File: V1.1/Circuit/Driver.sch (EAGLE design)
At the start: 25 parts, among them IC1 DRV8300DIPWR

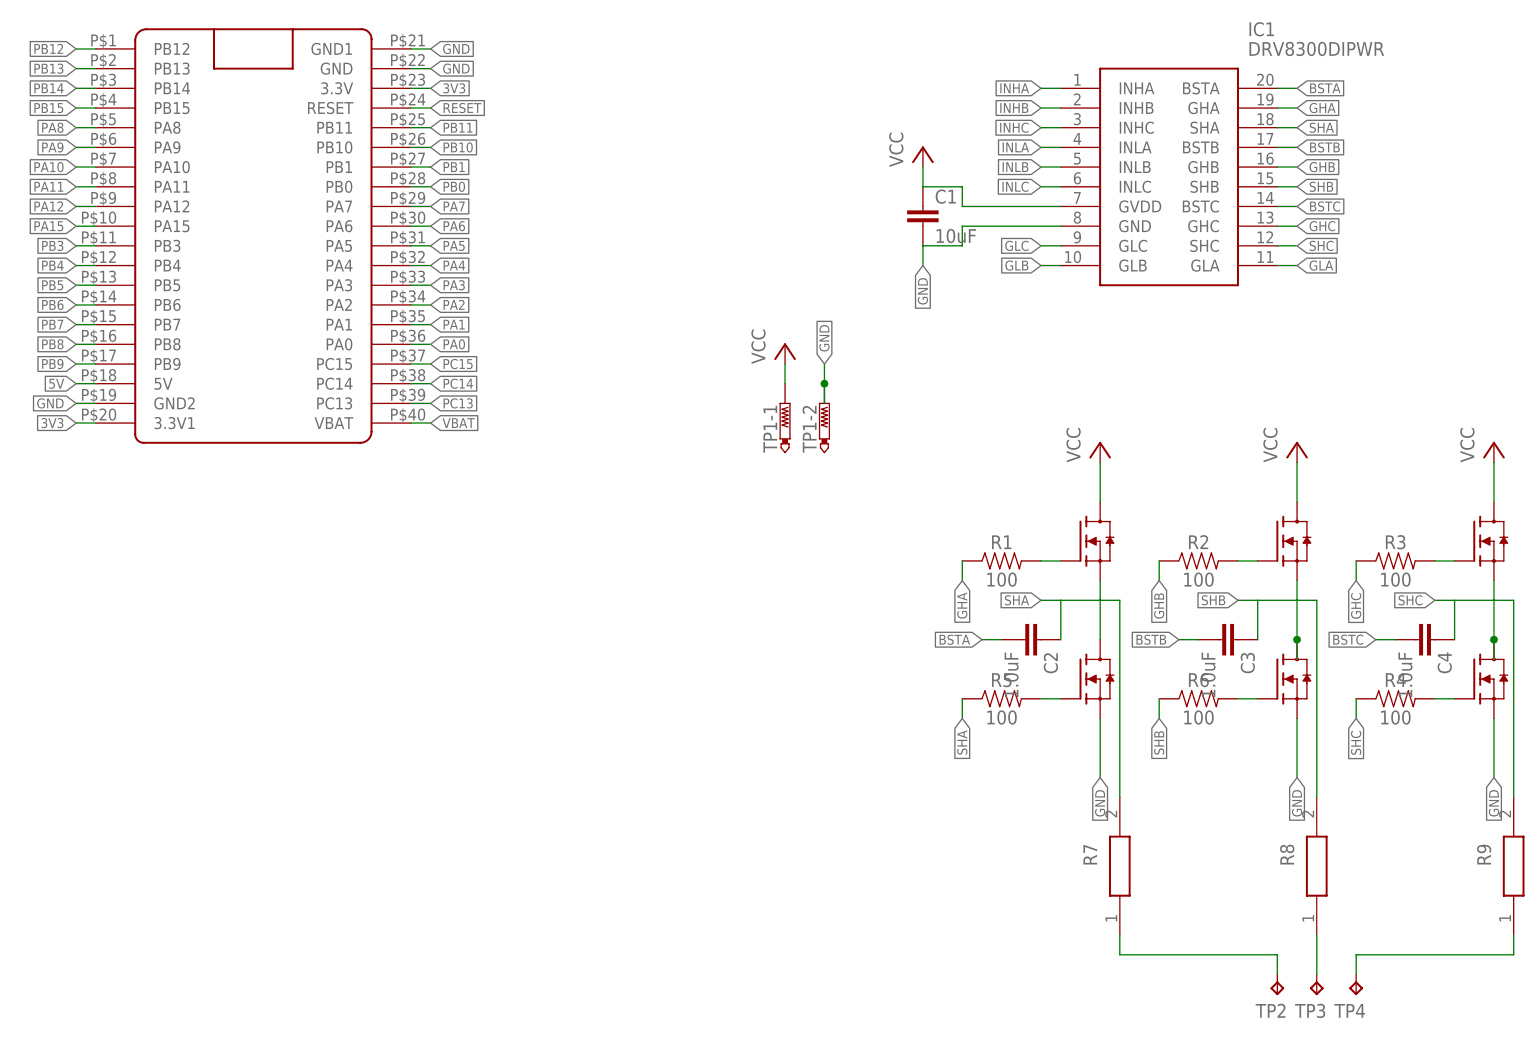
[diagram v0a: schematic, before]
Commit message: Added the FOC library
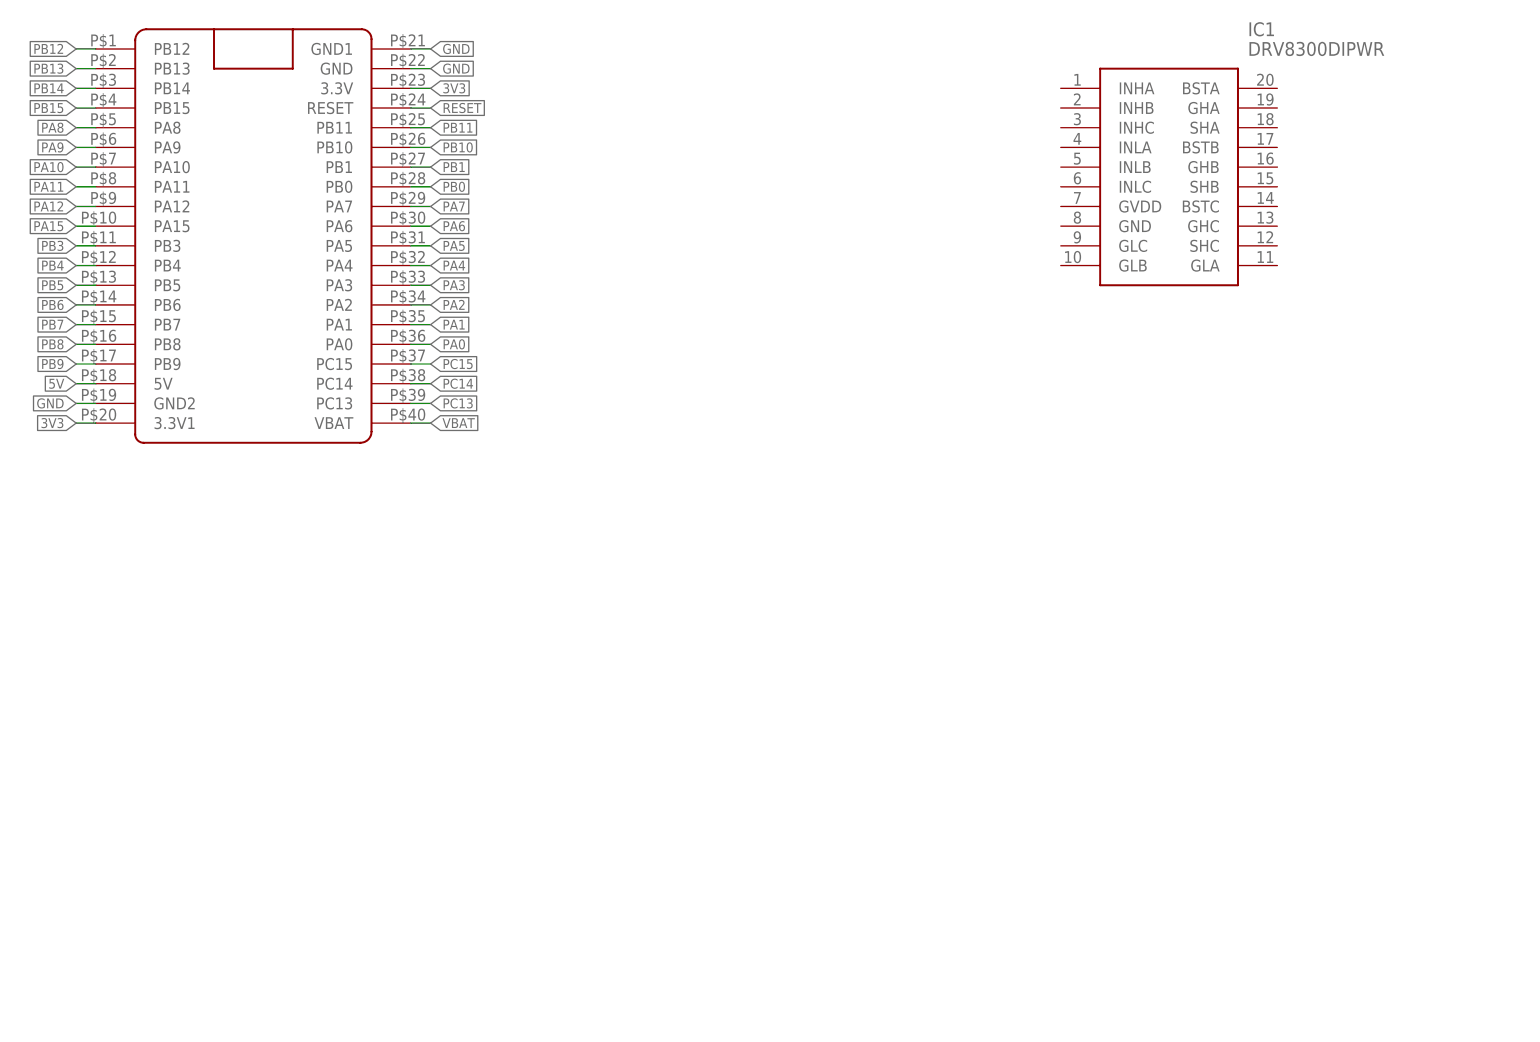
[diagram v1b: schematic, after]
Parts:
- removed C1: 10uF, SparkFun-Capacitors:10UF-0603-6.3V-20%
- removed C2, C3, C4: 1.0uF, SparkFun-Capacitors:1.0UF-0603-16V-10%
- removed R1, R2, R3, R4, R5, R6: 100, SparkFun-Resistors:100OHM-0603-1/10W-1%
- removed R7, R8, R9: CR2512-FX-51R1ELF, CR2512-FX-51R1ELF:CR2512-FX-51R1ELF
- removed TP1: PTR2, testpad:PTR2
- removed TP2, TP3, TP4: TPTP20SQ, testpad:TPTP20SQ
- removed U$2, U$3, U$4, U$5, U$6, U$7: IRLR7843, BLDC project:IRLR7843
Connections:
- removed net BSTA: C2.2, IC1.BSTA
- removed net BSTB: C3.2, IC1.BSTB
- removed net BSTC: C4.2, IC1.BSTC
- removed net GHA: IC1.GHA, R1.1
- removed net GHB: IC1.GHB, R2.1
- removed net GHC: IC1.GHC, R3.1
- removed net GLA: IC1.GLA
- removed net GLB: IC1.GLB
- removed net GLC: IC1.GLC
- removed net INHA: IC1.INHA
- removed net INHB: IC1.INHB
- removed net INHC: IC1.INHC
- removed net INLA: IC1.INLA
- removed net INLB: IC1.INLB
- removed net INLC: IC1.INLC
- removed net N$1: R1.2, U$2.G
- removed net N$2: R2.2, U$4.G
- removed net N$3: R3.2, U$6.G
- removed net N$4: R5.2, U$3.G
- removed net N$5: R6.2, U$5.G
- removed net N$6: R4.2, U$7.G
- removed net N$7: R7.1, TP2.TP
- removed net N$8: R8.1, TP3.TP
- removed net N$9: R9.1, TP4.TP
- removed net SHA: C2.1, IC1.SHA, R5.1, R7.2, U$2.S, U$3.D
- removed net SHB: C3.1, IC1.SHB, R6.1, R8.2, U$4.S, U$5.D
- removed net SHC: C4.1, IC1.SHC, R4.1, R9.2, U$6.S, U$7.D
- removed net VCC: C1.1, IC1.GVDD, TP1-1.TP, U$2.D, U$4.D, U$6.D
- net GND: no longer C1.2, IC1.GND, TP1-2.TP, U$3.S, U$5.S, U$7.S

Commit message: Circuit: Added DRV8300, and the Gate Circuit. Haven't added the Not gate
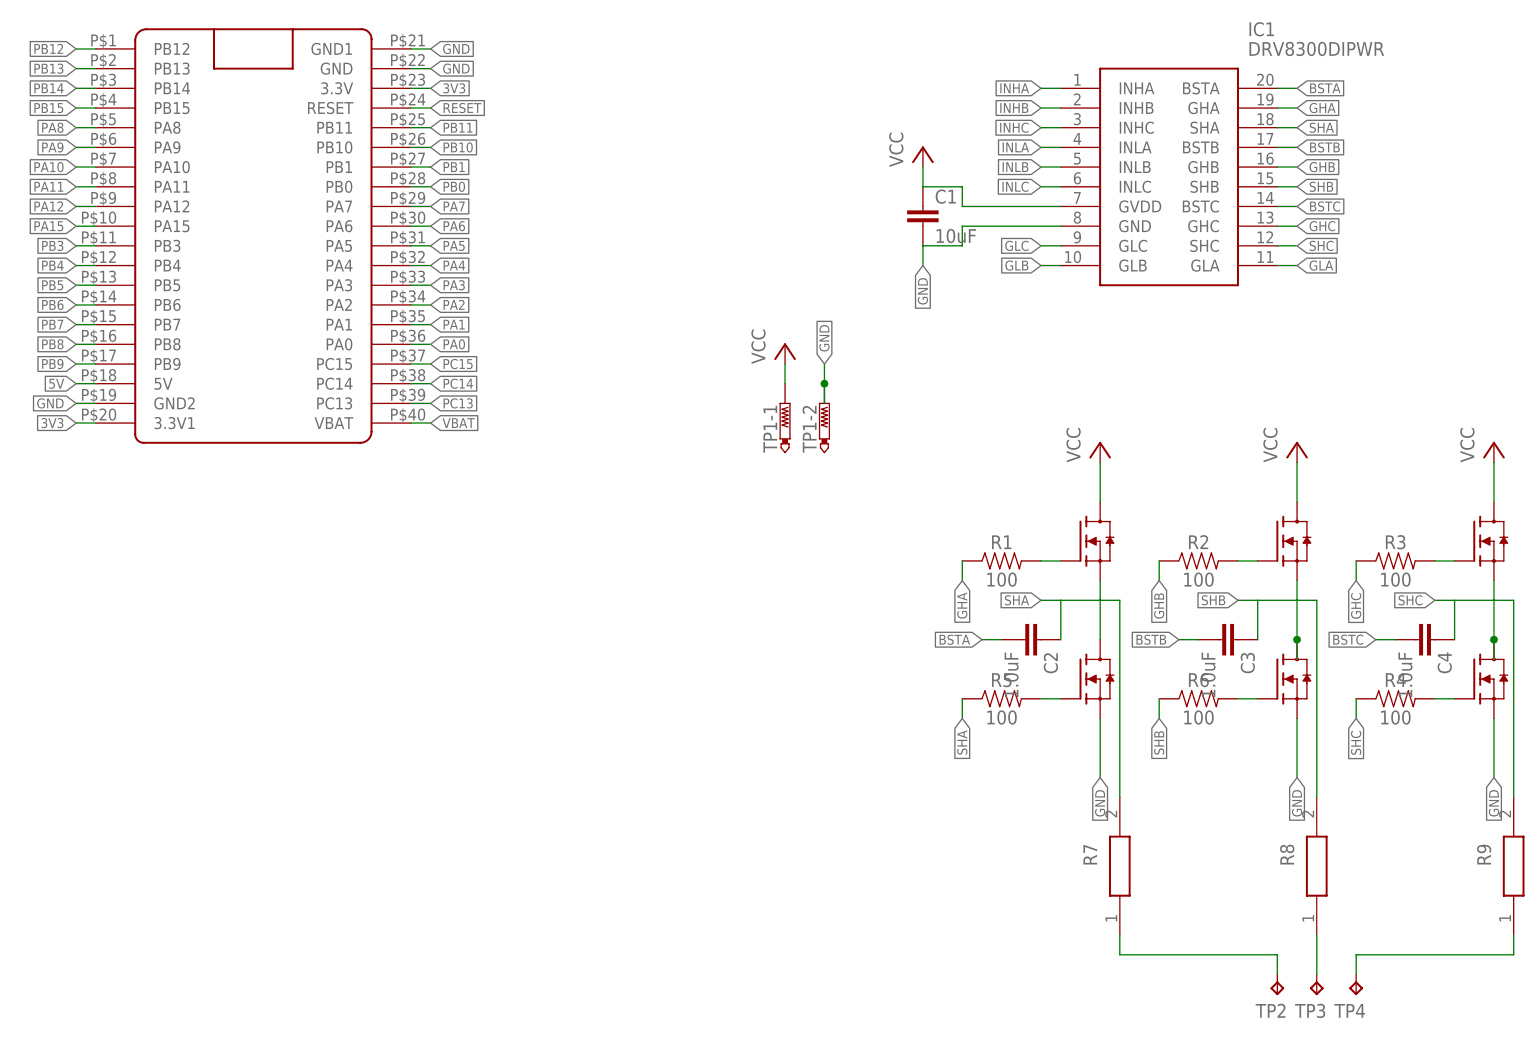
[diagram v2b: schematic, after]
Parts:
- added C1: 10uF, SparkFun-Capacitors:10UF-0603-6.3V-20%
- added C2, C3, C4: 1.0uF, SparkFun-Capacitors:1.0UF-0603-16V-10%
- added R1, R2, R3, R4, R5, R6: 100, SparkFun-Resistors:100OHM-0603-1/10W-1%
- added R7, R8, R9: CR2512-FX-51R1ELF, CR2512-FX-51R1ELF:CR2512-FX-51R1ELF
- added TP1: PTR2, testpad:PTR2
- added TP2, TP3, TP4: TPTP20SQ, testpad:TPTP20SQ
- added U$2, U$3, U$4, U$5, U$6, U$7: IRLR7843, BLDC project:IRLR7843
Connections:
- new net BSTA: C2.2, IC1.BSTA
- new net BSTB: C3.2, IC1.BSTB
- new net BSTC: C4.2, IC1.BSTC
- new net GHA: IC1.GHA, R1.1
- new net GHB: IC1.GHB, R2.1
- new net GHC: IC1.GHC, R3.1
- new net GLA: IC1.GLA
- new net GLB: IC1.GLB
- new net GLC: IC1.GLC
- new net INHA: IC1.INHA
- new net INHB: IC1.INHB
- new net INHC: IC1.INHC
- new net INLA: IC1.INLA
- new net INLB: IC1.INLB
- new net INLC: IC1.INLC
- new net N$1: R1.2, U$2.G
- new net N$2: R2.2, U$4.G
- new net N$3: R3.2, U$6.G
- new net N$4: R5.2, U$3.G
- new net N$5: R6.2, U$5.G
- new net N$6: R4.2, U$7.G
- new net N$7: R7.1, TP2.TP
- new net N$8: R8.1, TP3.TP
- new net N$9: R9.1, TP4.TP
- new net SHA: C2.1, IC1.SHA, R5.1, R7.2, U$2.S, U$3.D
- new net SHB: C3.1, IC1.SHB, R6.1, R8.2, U$4.S, U$5.D
- new net SHC: C4.1, IC1.SHC, R4.1, R9.2, U$6.S, U$7.D
- new net VCC: C1.1, IC1.GVDD, TP1-1.TP, U$2.D, U$4.D, U$6.D
- net GND: now also C1.2, IC1.GND, TP1-2.TP, U$3.S, U$5.S, U$7.S
